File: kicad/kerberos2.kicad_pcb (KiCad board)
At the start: 2 copper layers, 62.5 x 83.8 mm, 15 parts, among them J1 USB4125-GF-A_REVA2, J2 MIDI-in, J3 MIDI-thru, J4 MIDI-out, SW1 TL1105JAF160Q, U1 RP2040, U2 W9812G6KH-6, U3 T8Q144, U4 MX25L25645G

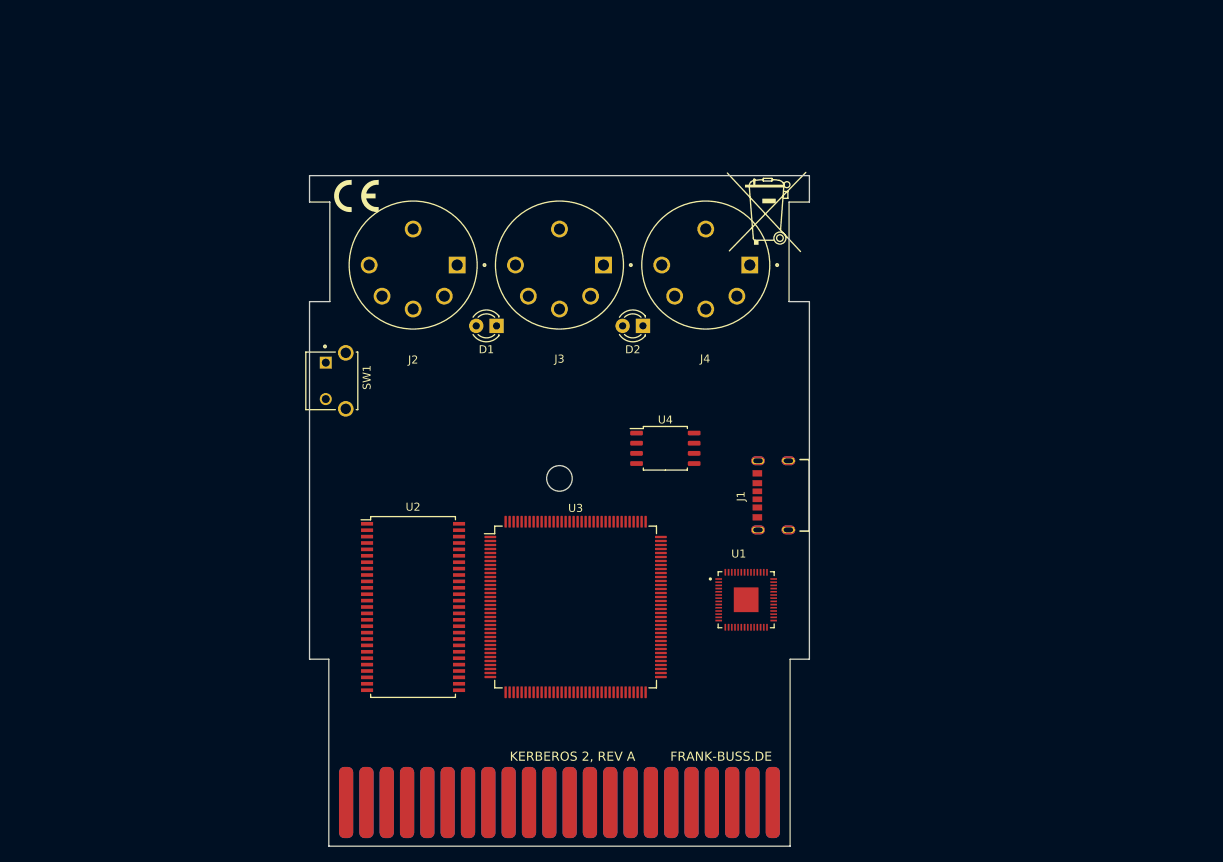
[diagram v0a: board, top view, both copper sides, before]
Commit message: first complete test version for Kerberos 2
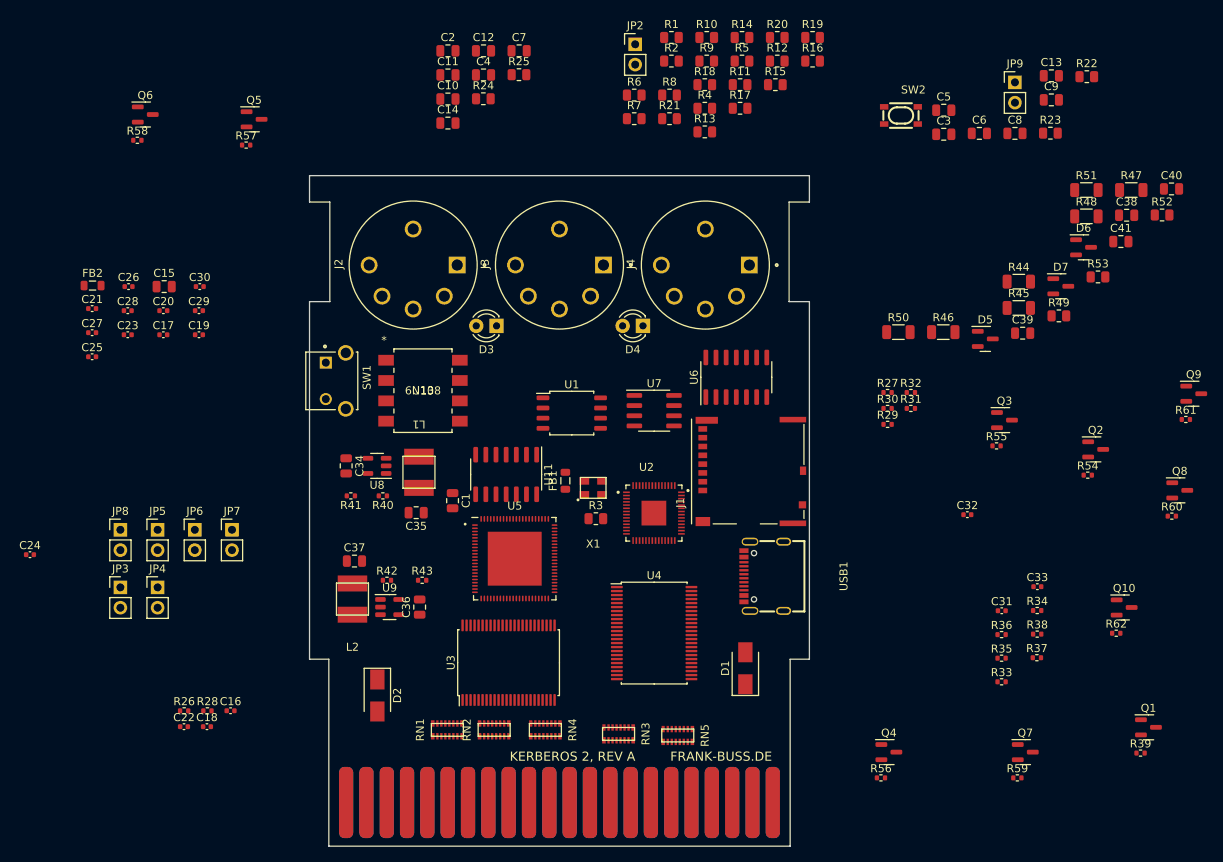
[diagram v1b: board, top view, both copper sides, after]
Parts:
- removed @HOLE0: , 
- removed U$1: , midi:CE-4MM
- removed U$2: , midi:MUELLTONNE_10.00
- removed the U1 at (100.4, 92.0)
- added C1: 100n, Capacitor_SMD:C_0805_2012Metric, F.Cu at (63.7, 79.7)
- added C10: 100n, Capacitor_SMD:C_0805_2012Metric, F.Cu at (63.1, 29.4)
- added C11: 100n, Capacitor_SMD:C_0805_2012Metric, F.Cu at (63.1, 26.4)
- added C12: 100n, Capacitor_SMD:C_0805_2012Metric, F.Cu at (67.6, 23.4)
- added C13: 100n, Capacitor_SMD:C_0805_2012Metric, F.Cu at (138.6, 26.5)
- added C14: 1u, Capacitor_SMD:C_0805_2012Metric, F.Cu at (63.1, 32.5)
- added C15: 4.7u, Capacitor_SMD:C_0805_2012Metric, F.Cu at (27.6, 52.9)
- added C16: 100n, Capacitor_SMD:C_0402_1005Metric, F.Cu at (36.0, 105.9)
- added C17: 100n, Capacitor_SMD:C_0402_1005Metric, F.Cu at (27.6, 58.9)
- added C18: 100n, Capacitor_SMD:C_0402_1005Metric, F.Cu at (33.0, 107.9)
- added C19: 100n, Capacitor_SMD:C_0402_1005Metric, F.Cu at (32.0, 58.9)
- added C2: 10u, Capacitor_SMD:C_0805_2012Metric, F.Cu at (63.1, 23.4)
- added C20: 100n, Capacitor_SMD:C_0402_1005Metric, F.Cu at (27.6, 55.9)
- added C21: 100n, Capacitor_SMD:C_0402_1005Metric, F.Cu at (18.6, 55.6)
- added C22: 100n, Capacitor_SMD:C_0402_1005Metric, F.Cu at (30.1, 107.9)
- added C23: 100n, Capacitor_SMD:C_0402_1005Metric, F.Cu at (23.1, 58.9)
- added C24: 100n, Capacitor_SMD:C_0402_1005Metric, F.Cu at (10.9, 86.4)
- added C25: 100n, Capacitor_SMD:C_0402_1005Metric, F.Cu at (18.6, 61.7)
- added C26: 100n, Capacitor_SMD:C_0402_1005Metric, F.Cu at (23.2, 52.9)
- added C27: 100n, Capacitor_SMD:C_0402_1005Metric, F.Cu at (18.6, 58.6)
- added C28: 100n, Capacitor_SMD:C_0402_1005Metric, F.Cu at (23.1, 55.9)
- added C29: 100n, Capacitor_SMD:C_0402_1005Metric, F.Cu at (32.0, 55.9)
- added C3: 100n, Capacitor_SMD:C_0805_2012Metric, F.Cu at (125.1, 33.9)
- added C30: 100n, Capacitor_SMD:C_0402_1005Metric, F.Cu at (32.1, 52.9)
- added C31: 100n, Capacitor_SMD:C_0402_1005Metric, F.Cu at (132.3, 93.4)
- added C32: 100n, Capacitor_SMD:C_0402_1005Metric, F.Cu at (128.1, 81.4)
- added C33: 100n, Capacitor_SMD:C_0402_1005Metric, F.Cu at (136.8, 90.4)
- added C34: 4.7u, Capacitor_SMD:C_0805_2012Metric, F.Cu at (50.4, 75.3)
- added C35: 10u, Capacitor_SMD:C_0805_2012Metric, F.Cu at (59.1, 81.2)
- added C36: 4.7u, Capacitor_SMD:C_0805_2012Metric, F.Cu at (59.6, 93.0)
- added C37: 10u, Capacitor_SMD:C_0805_2012Metric, F.Cu at (51.4, 87.2)
- added C38: 1n, Capacitor_SMD:C_0805_2012Metric, F.Cu at (148.0, 44.0)
- added C39: 1n, Capacitor_SMD:C_0805_2012Metric, F.Cu at (135.0, 58.7)
- added C4: 100n, Capacitor_SMD:C_0805_2012Metric, F.Cu at (67.6, 26.4)
- added C40: 100n, Capacitor_SMD:C_0805_2012Metric, F.Cu at (153.6, 40.7)
- added C41: 100n, Capacitor_SMD:C_0805_2012Metric, F.Cu at (147.2, 47.3)
- added C5: 100n, Capacitor_SMD:C_0805_2012Metric, F.Cu at (125.1, 30.8)
- added C6: 100n, Capacitor_SMD:C_0805_2012Metric, F.Cu at (129.6, 33.7)
- added C7: 100n, Capacitor_SMD:C_0805_2012Metric, F.Cu at (72.0, 23.4)
- added C8: 100n, Capacitor_SMD:C_0805_2012Metric, F.Cu at (134.0, 33.7)
- added C9: 1u, Capacitor_SMD:C_0805_2012Metric, F.Cu at (138.6, 29.6)
- added D3: ~, LED_THT:LED_D3.0mm, F.Cu at (69.2, 57.8)
- added D4: ~, LED_THT:LED_D3.0mm, F.Cu at (87.5, 57.8)
- added D5: BAV99, Package_TO_SOT_SMD:SOT-23, F.Cu at (130.3, 59.4)
- added D6: BAV99, Package_TO_SOT_SMD:SOT-23, F.Cu at (142.6, 48.0)
- added D7: BAV99, Package_TO_SOT_SMD:SOT-23, F.Cu at (139.7, 52.9)
- added FB1: FerriteBead, Inductor_SMD:L_0805_2012Metric, F.Cu at (77.8, 77.2)
- added FB2: FerriteBead, Inductor_SMD:L_0805_2012Metric, F.Cu at (18.7, 52.8)
- added JP2: host-mode-supply, Connector_PinHeader_2.54mm:PinHeader_1x02_P2.54mm_Vertical, F.Cu at (86.5, 22.6)
- added JP3: 3.3V+, Connector_PinHeader_2.54mm:PinHeader_1x02_P2.54mm_Vertical, F.Cu at (22.2, 90.5)
- added JP4: 3.3V, Connector_PinHeader_2.54mm:PinHeader_1x02_P2.54mm_Vertical, F.Cu at (26.8, 90.5)
- added JP5: 3.3V-, Connector_PinHeader_2.54mm:PinHeader_1x02_P2.54mm_Vertical, F.Cu at (26.8, 83.3)
- added JP6: 1.2V+, Connector_PinHeader_2.54mm:PinHeader_1x02_P2.54mm_Vertical, F.Cu at (31.5, 83.3)
- added JP7: 1.2V, Connector_PinHeader_2.54mm:PinHeader_1x02_P2.54mm_Vertical, F.Cu at (36.1, 83.3)
- added JP8: 1.2V-, Connector_PinHeader_2.54mm:PinHeader_1x02_P2.54mm_Vertical, F.Cu at (22.2, 83.3)
- added JP9: ~{USB_BOOT}, Connector_PinHeader_2.54mm:PinHeader_1x02_P2.54mm_Vertical, F.Cu at (134.0, 27.4)
- added L1: 4.7u, coil:coil, F.Cu at (59.5, 76.1)
- added L2: 4.7u, coil:coil, F.Cu at (51.2, 92.0)
- added Q1: Q_NMOS_GSD, Package_TO_SOT_SMD:SOT-23, F.Cu at (150.7, 108.0)
- added Q10: Q_NMOS_GSD, Package_TO_SOT_SMD:SOT-23, F.Cu at (147.7, 93.0)
- added Q2: Q_NMOS_GSD, Package_TO_SOT_SMD:SOT-23, F.Cu at (144.1, 73.2)
- added Q3: Q_NMOS_GSD, Package_TO_SOT_SMD:SOT-23, F.Cu at (132.7, 69.6)
- added Q4: Q_NMOS_GSD, Package_TO_SOT_SMD:SOT-23, F.Cu at (118.2, 111.1)
- added Q5: Q_NMOS_GSD, Package_TO_SOT_SMD:SOT-23, F.Cu at (38.9, 32.0)
- added Q6: Q_NMOS_GSD, Package_TO_SOT_SMD:SOT-23, F.Cu at (25.3, 31.4)
- added Q7: Q_NMOS_GSD, Package_TO_SOT_SMD:SOT-23, F.Cu at (135.3, 111.1)
- added Q8: Q_NMOS_GSD, Package_TO_SOT_SMD:SOT-23, F.Cu at (154.6, 78.4)
- added Q9: Q_NMOS_GSD, Package_TO_SOT_SMD:SOT-23, F.Cu at (156.3, 66.3)
- added R1: 5.1, Resistor_SMD:R_0805_2012Metric, F.Cu at (91.1, 21.8)
- added R10: 22, Resistor_SMD:R_0805_2012Metric, F.Cu at (95.5, 21.8)
- added R11: 22, Resistor_SMD:R_0805_2012Metric, F.Cu at (99.6, 27.6)
- added R12: 22, Resistor_SMD:R_0805_2012Metric, F.Cu at (104.3, 24.7)
- added R13: 22, Resistor_SMD:R_0805_2012Metric, F.Cu at (95.2, 33.5)
- added R14: 22, Resistor_SMD:R_0805_2012Metric, F.Cu at (99.9, 21.8)
- added R15: 22, Resistor_SMD:R_0805_2012Metric, F.Cu at (104.0, 27.6)
- added R16: 22, Resistor_SMD:R_0805_2012Metric, F.Cu at (108.7, 24.7)
- added R17: 22, Resistor_SMD:R_0805_2012Metric, F.Cu at (99.6, 30.6)
- added R18: 22, Resistor_SMD:R_0805_2012Metric, F.Cu at (95.2, 27.6)
- added R19: 22, Resistor_SMD:R_0805_2012Metric, F.Cu at (108.7, 21.8)
- added R2: 5.1, Resistor_SMD:R_0805_2012Metric, F.Cu at (91.1, 24.7)
- added R20: 1k, Resistor_SMD:R_0805_2012Metric, F.Cu at (104.3, 21.8)
- added R21: 1k, Resistor_SMD:R_0805_2012Metric, F.Cu at (90.8, 31.9)
- added R22: 10k, Resistor_SMD:R_0805_2012Metric, F.Cu at (143.0, 26.6)
- added R23: 10k, Resistor_SMD:R_0805_2012Metric, F.Cu at (138.4, 33.7)
- added R24: 1k, Resistor_SMD:R_0805_2012Metric, F.Cu at (67.5, 29.4)
- added R25: 10k, Resistor_SMD:R_0805_2012Metric, F.Cu at (72.0, 26.4)
- added R26: 10k, Resistor_SMD:R_0402_1005Metric, F.Cu at (30.1, 105.9)
- added R27: 10k, Resistor_SMD:R_0402_1005Metric, F.Cu at (118.1, 66.1)
- added R28: 10k, Resistor_SMD:R_0402_1005Metric, F.Cu at (33.1, 105.9)
- added R29: 10k, Resistor_SMD:R_0402_1005Metric, F.Cu at (118.1, 70.1)
- added R3: 27, Resistor_SMD:R_0805_2012Metric, F.Cu at (81.6, 81.9)
- added R30: 10k, Resistor_SMD:R_0402_1005Metric, F.Cu at (118.1, 68.1)
- added R31: 10k, Resistor_SMD:R_0402_1005Metric, F.Cu at (121.0, 68.1)
- added R32: 10k, Resistor_SMD:R_0402_1005Metric, F.Cu at (121.0, 66.1)
- added R33: 10k, Resistor_SMD:R_0402_1005Metric, F.Cu at (132.3, 102.3)
- added R34: 10k, Resistor_SMD:R_0402_1005Metric, F.Cu at (136.8, 93.4)
- added R35: 1k, Resistor_SMD:R_0402_1005Metric, F.Cu at (132.3, 99.3)
- added R36: 1k, Resistor_SMD:R_0402_1005Metric, F.Cu at (132.3, 96.4)
- added R37: 10k, Resistor_SMD:R_0402_1005Metric, F.Cu at (136.7, 99.3)
- added R38: 10k, Resistor_SMD:R_0402_1005Metric, F.Cu at (136.8, 96.3)
- added R39: 10k, Resistor_SMD:R_0402_1005Metric, F.Cu at (149.7, 111.2)
- added R4: 27, Resistor_SMD:R_0805_2012Metric, F.Cu at (95.2, 30.6)
- added R40: R, Resistor_SMD:R_0402_1005Metric, F.Cu at (55.0, 79.0)
- added R41: R, Resistor_SMD:R_0402_1005Metric, F.Cu at (51.0, 79.0)
- added R42: R, Resistor_SMD:R_0402_1005Metric, F.Cu at (55.5, 89.6)
- added R43: R, Resistor_SMD:R_0402_1005Metric, F.Cu at (59.9, 89.6)
- added R44: 220, Resistor_SMD:R_1206_3216Metric, F.Cu at (134.5, 52.3)
- added R45: 220, Resistor_SMD:R_1206_3216Metric, F.Cu at (134.5, 55.6)
- added R46: 220, Resistor_SMD:R_1206_3216Metric, F.Cu at (125.0, 58.6)
- added R47: 220, Resistor_SMD:R_1206_3216Metric, F.Cu at (148.5, 40.8)
- added R48: 220, Resistor_SMD:R_1206_3216Metric, F.Cu at (142.9, 44.1)
- added R49: 10k, Resistor_SMD:R_0805_2012Metric, F.Cu at (139.5, 56.5)
- added R5: 27, Resistor_SMD:R_0805_2012Metric, F.Cu at (99.9, 24.7)
- added R50: 220, Resistor_SMD:R_1206_3216Metric, F.Cu at (119.4, 58.6)
- added R51: 220, Resistor_SMD:R_1206_3216Metric, F.Cu at (142.9, 40.8)
- added R52: 1k8, Resistor_SMD:R_0805_2012Metric, F.Cu at (152.4, 43.9)
- added R53: 3k3, Resistor_SMD:R_0805_2012Metric, F.Cu at (144.4, 51.7)
- added R54: 10k, Resistor_SMD:R_0402_1005Metric, F.Cu at (143.1, 76.5)
- added R55: 10k, Resistor_SMD:R_0402_1005Metric, F.Cu at (131.7, 72.8)
- added R56: 10k, Resistor_SMD:R_0402_1005Metric, F.Cu at (117.2, 114.3)
- added R57: 10k, Resistor_SMD:R_0402_1005Metric, F.Cu at (37.9, 35.2)
- added R58: 10k, Resistor_SMD:R_0402_1005Metric, F.Cu at (24.3, 34.6)
- added R59: 10k, Resistor_SMD:R_0402_1005Metric, F.Cu at (134.3, 114.3)
- added R6: 27, Resistor_SMD:R_0805_2012Metric, F.Cu at (86.4, 28.9)
- added R60: 10k, Resistor_SMD:R_0402_1005Metric, F.Cu at (153.6, 81.6)
- added R61: 10k, Resistor_SMD:R_0402_1005Metric, F.Cu at (155.4, 69.5)
- added R62: 10k, Resistor_SMD:R_0402_1005Metric, F.Cu at (146.7, 96.2)
- added R7: 22, Resistor_SMD:R_0805_2012Metric, F.Cu at (86.4, 31.9)
- added R8: 22, Resistor_SMD:R_0805_2012Metric, F.Cu at (90.8, 28.9)
- added R9: 22, Resistor_SMD:R_0805_2012Metric, F.Cu at (95.5, 24.7)
- added RN1: 33, resistor-network:16P8, F.Cu at (63.0, 108.3)
- added RN2: 33, resistor-network:16P8, F.Cu at (68.9, 108.3)
- added RN3: 33, resistor-network:16P8, F.Cu at (84.5, 108.8)
- added RN4: 33, resistor-network:16P8, F.Cu at (75.3, 108.3)
- added RN5: 33, resistor-network:16P8, F.Cu at (91.8, 109.0)
- added SW2: SKRPADE010, button:KEY-SMD_4P-L4.2-W3.2-P2.20-LS4.6, F.Cu at (119.8, 31.5)
- added U10: 6N138, 6N138S:6N138S, F.Cu at (60.0, 65.9)
- added U11: 74LS14, Package_SO:SOIC-14_3.9x8.7mm_P1.27mm, F.Cu at (70.4, 76.4)
- added U4: 74ALVC164245DGG,51, Package_SO:TSSOP-48_8x12.5mm_P0.5mm, F.Cu at (88.9, 96.2)
- added U5: GW1NR-4&4B_QN881, qn88:QFN-88_EP_10x10_Pitch0.4mm, F.Cu at (71.5, 86.9)
- added U6: AD8694ARZ, Package_SO:SOIC-14_3.9x8.7mm_P1.27mm, F.Cu at (99.2, 64.2)
- added U7: TMCS1108A3UQDR, Package_SO:SOIC-8_3.9x4.9mm_P1.27mm, F.Cu at (88.9, 68.4)
- added U8: M3406, Package_TO_SOT_SMD:TSOT-23-5, F.Cu at (54.3, 75.3)
- added U9: M3406, Package_TO_SOT_SMD:TSOT-23-5, F.Cu at (55.8, 93.0)
- added USB1: TYPEC-304J-BCP16, usb-c:USB-C-SMD_TYPEC-304J-BCP16, F.Cu at (102.6, 89.1)
- added X1: SX3M12.000M20F30TNN, oscillator:SX3M12.000M20F30TNN, F.Cu at (81.3, 78.0)
- D1, D2: value LED -> D_Schottky; footprint LED_THT:LED_D3.0mm -> Diode_SMD:D_SMA
- J1: value USB4125-GF-A_REVA2 -> 503398-1892; footprint usb-c:GCT_USB4125-GF-A_REVA2 -> sd-card:MOLEX_503398-1892
- SW1: value TL1105JAF160Q -> side-button
- U2: value W9812G6KH-6 -> RP2040; footprint Package_SO:TSOP-II-54_22.2x10.16mm_P0.8mm -> rp2040:QFN40P700X700X90-57N
- U3: value T8Q144 -> 74ALVC164245DGG,51; footprint Package_QFP:LQFP-144_20x20mm_P0.5mm -> Package_SO:TSSOP-48_8x12.5mm_P0.5mm
- moved D2 56.9 mm to (54.3, 104.0), turned to -90 degrees
- moved D1 52.9 mm to (100.3, 100.6), turned to 90 degrees
- moved U2 32.3 mm to (88.9, 81.2)
- moved U1 12.5 mm to (78.6, 68.7)
- moved U3 10.9 mm to (70.7, 99.9), turned to 90 degrees
- moved J1 5.22 mm to (100.6, 76.0)
- moved J4 0.05 mm to (95.3, 50.2)
- renumbered U4 to U1
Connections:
- D1 pad 1: unconnected-(D1-Pad1) -> +5V
- D1 pad 2: unconnected-(D1-Pad2) -> Net-(D1-Pad2)
- D2 pad 1: unconnected-(D2-Pad1) -> +5V
- D2 pad 2: unconnected-(D2-Pad2) -> Net-(D2-Pad2)
- J2 pad 4: unconnected-(J2-Pad4) -> Net-(J2-Pad4)
- J2 pad 5: unconnected-(J2-Pad5) -> Net-(D5-Pad1)
- J3 pad 2: unconnected-(J3-Pad2) -> GND
- J3 pad 4: unconnected-(J3-Pad4) -> Net-(J3-Pad4)
- J3 pad 5: unconnected-(J3-Pad5) -> Net-(C38-Pad1)
- J3 pad S: unconnected-(J3-PadS) -> GND
- J4 pad 2: unconnected-(J4-Pad2) -> GND
- J4 pad 4: unconnected-(J4-Pad4) -> Net-(J4-Pad4)
- J4 pad 5: unconnected-(J4-Pad5) -> Net-(C39-Pad1)
- J4 pad S: unconnected-(J4-PadS) -> GND
- JP1 pad 1: unconnected-(JP1-Pad1) -> GND
- JP1 pad 10: unconnected-(JP1-Pad10) -> Net-(JP1-Pad10)
- JP1 pad 11: unconnected-(JP1-Pad11) -> Net-(JP1-Pad11)
- JP1 pad 12: unconnected-(JP1-Pad12) -> Net-(JP1-Pad12)
- JP1 pad 13: unconnected-(JP1-Pad13) -> Net-(JP1-Pad13)
- JP1 pad 14: unconnected-(JP1-Pad14) -> Net-(JP1-Pad14)
- JP1 pad 15: unconnected-(JP1-Pad15) -> Net-(JP1-Pad15)
- JP1 pad 16: unconnected-(JP1-Pad16) -> Net-(JP1-Pad16)
- JP1 pad 17: unconnected-(JP1-Pad17) -> Net-(JP1-Pad17)
- JP1 pad 18: unconnected-(JP1-Pad18) -> Net-(JP1-Pad18)
- JP1 pad 19: unconnected-(JP1-Pad19) -> Net-(JP1-Pad19)
- JP1 pad 2: unconnected-(JP1-Pad2) -> Net-(D2-Pad2)
- JP1 pad 20: unconnected-(JP1-Pad20) -> Net-(JP1-Pad20)
- JP1 pad 21: unconnected-(JP1-Pad21) -> Net-(JP1-Pad21)
- JP1 pad 22: unconnected-(JP1-Pad22) -> GND
- JP1 pad 3: unconnected-(JP1-Pad3) -> Net-(D2-Pad2)
- JP1 pad 4: unconnected-(JP1-Pad4) -> Net-(JP1-Pad4)
- JP1 pad 5: unconnected-(JP1-Pad5) -> Net-(JP1-Pad5)
- JP1 pad 6: unconnected-(JP1-Pad6) -> Net-(JP1-Pad6)
- JP1 pad 7: unconnected-(JP1-Pad7) -> Net-(JP1-Pad7)
- JP1 pad 8: unconnected-(JP1-Pad8) -> Net-(JP1-Pad8)
- JP1 pad 9: unconnected-(JP1-Pad9) -> Net-(JP1-Pad9)
- JP1 pad A: unconnected-(JP1-PadA) -> GND
- JP1 pad B: unconnected-(JP1-PadB) -> Net-(JP1-PadB)
- JP1 pad C: unconnected-(JP1-PadC) -> Net-(JP1-PadC)
- JP1 pad D: unconnected-(JP1-PadD) -> Net-(JP1-PadD)
- JP1 pad E: unconnected-(JP1-PadE) -> Net-(JP1-PadE)
- JP1 pad F: unconnected-(JP1-PadF) -> Net-(JP1-PadF)
- JP1 pad H: unconnected-(JP1-PadH) -> Net-(JP1-PadH)
- JP1 pad J: unconnected-(JP1-PadJ) -> Net-(JP1-PadJ)
- JP1 pad K: unconnected-(JP1-PadK) -> Net-(JP1-PadK)
- JP1 pad L: unconnected-(JP1-PadL) -> Net-(JP1-PadL)
- JP1 pad M: unconnected-(JP1-PadM) -> Net-(JP1-PadM)
- JP1 pad N: unconnected-(JP1-PadN) -> Net-(JP1-PadN)
- JP1 pad P: unconnected-(JP1-PadP) -> Net-(JP1-PadP)
- JP1 pad R: unconnected-(JP1-PadR) -> Net-(JP1-PadR)
- JP1 pad S: unconnected-(JP1-PadS) -> Net-(JP1-PadS)
- JP1 pad T: unconnected-(JP1-PadT) -> Net-(JP1-PadT)
- JP1 pad U: unconnected-(JP1-PadU) -> Net-(JP1-PadU)
- JP1 pad V: unconnected-(JP1-PadV) -> Net-(JP1-PadV)
- JP1 pad W: unconnected-(JP1-PadW) -> Net-(JP1-PadW)
- JP1 pad X: unconnected-(JP1-PadX) -> Net-(JP1-PadX)
- JP1 pad Y: unconnected-(JP1-PadY) -> Net-(JP1-PadY)
- JP1 pad Z: unconnected-(JP1-PadZ) -> GND
- SW1 pad 1: unconnected-(SW1-Pad1) -> GND
- SW1 pad 2: unconnected-(SW1-Pad2) -> Net-(R22-Pad2)
- U1 pad 1: unconnected-(U4-Pad1) -> /GW1NR FPGA/FLASH_CS
- U1 pad 2: unconnected-(U4-Pad2) -> /GW1NR FPGA/FLASH-SIO1
- U1 pad 3: unconnected-(U4-Pad3) -> /GW1NR FPGA/FLASH-SIO2
- U1 pad 4: unconnected-(U4-Pad4) -> GND
- U1 pad 5: unconnected-(U4-Pad5) -> /GW1NR FPGA/FLASH-SIO0
- U1 pad 6: unconnected-(U4-Pad6) -> /GW1NR FPGA/FLASH-SCLK
- U1 pad 7: unconnected-(U4-Pad7) -> /GW1NR FPGA/FLASH-SIO3
- U1 pad 8: unconnected-(U4-Pad8) -> +3.3V
- U2 pad 1: Net-(U2-Pad1) -> +3.3V
- U2 pad 10: unconnected-(U2-Pad10) -> +3.3V
- U2 pad 11: unconnected-(U2-Pad11) -> /RP2040 microcontroller/spare2
- U2 pad 12: Net-(U2-Pad12) -> /RP2040 microcontroller/spare3
- U2 pad 13: unconnected-(U2-Pad13) -> /RP2040 microcontroller/spare4
- U2 pad 14: Net-(U2-Pad1) -> /RP2040 microcontroller/spare5
- U2 pad 15: unconnected-(U2-Pad15) -> /RP2040 microcontroller/spare6
- U2 pad 16: unconnected-(U2-Pad16) -> Net-(R22-Pad2)
- U2 pad 19: unconnected-(U2-Pad19) -> GND
- U2 pad 2: unconnected-(U2-Pad2) -> /RP2040 microcontroller/JTAGSEL_N
- U2 pad 20: unconnected-(U2-Pad20) -> /RP2040 microcontroller/XIN
- U2 pad 22: unconnected-(U2-Pad22) -> +3.3V
- U2 pad 23: unconnected-(U2-Pad23) -> /RP2040 microcontroller/1.1V
- U2 pad 26: unconnected-(U2-Pad26) -> Net-(R23-Pad1)
- U2 pad 27: Net-(U2-Pad1) -> unconnected-(U2-Pad27)
- U2 pad 28: Net-(U2-Pad28) -> unconnected-(U2-Pad28)
- U2 pad 3: Net-(U2-Pad3) -> /RP2040 microcontroller/TCK
- U2 pad 30: unconnected-(U2-Pad30) -> Net-(J1-Pad3)
- U2 pad 31: unconnected-(U2-Pad31) -> Net-(J1-Pad5)
- U2 pad 32: unconnected-(U2-Pad32) -> Net-(J1-Pad7)
- U2 pad 33: unconnected-(U2-Pad33) -> +3.3V
- U2 pad 34: unconnected-(U2-Pad34) -> Net-(J1-Pad8)
- U2 pad 35: unconnected-(U2-Pad35) -> Net-(J1-Pad1)
- U2 pad 36: unconnected-(U2-Pad36) -> Net-(J1-Pad2)
- U2 pad 37: unconnected-(U2-Pad37) -> Net-(J1-Pad10)
- U2 pad 4: unconnected-(U2-Pad4) -> /RP2040 microcontroller/TMS
- U2 pad 41: Net-(U2-Pad28) -> unconnected-(U2-Pad41)
- U2 pad 42: unconnected-(U2-Pad42) -> +3.3V
- U2 pad 43: Net-(U2-Pad3) -> +3.3V
- U2 pad 44: unconnected-(U2-Pad44) -> +3.3V
- U2 pad 45: unconnected-(U2-Pad45) -> /RP2040 microcontroller/1.1V
- U2 pad 46: Net-(U2-Pad12) -> /RP2040 microcontroller/USB_D-
- U2 pad 47: unconnected-(U2-Pad47) -> /RP2040 microcontroller/USB_D+
- U2 pad 48: unconnected-(U2-Pad48) -> +3.3V
- U2 pad 49: Net-(U2-Pad3) -> +3.3V
- U2 pad 5: unconnected-(U2-Pad5) -> /RP2040 microcontroller/TDO
- U2 pad 50: unconnected-(U2-Pad50) -> /RP2040 microcontroller/1.1V
- U2 pad 51: unconnected-(U2-Pad51) -> /GW1NR FPGA/FLASH-SIO3
- U2 pad 52: Net-(U2-Pad12) -> /GW1NR FPGA/FLASH-SCLK
- U2 pad 53: unconnected-(U2-Pad53) -> /GW1NR FPGA/FLASH-SIO0
- U2 pad 54: Net-(U2-Pad28) -> /GW1NR FPGA/FLASH-SIO2
- U2 pad 6: Net-(U2-Pad12) -> /RP2040 microcontroller/TDI
- U2 pad 7: unconnected-(U2-Pad7) -> /RP2040 microcontroller/DONE
- U2 pad 8: unconnected-(U2-Pad8) -> /RP2040 microcontroller/RECONFIG_N
- U2 pad 9: Net-(U2-Pad3) -> /RP2040 microcontroller/spare1
- U3 pad 1: unconnected-(U3-Pad1) -> /GW1NR FPGA/DIR_A
- U3 pad 10: unconnected-(U3-Pad10) -> GND
- U3 pad 11: unconnected-(U3-Pad11) -> /GW1NR FPGA/A6
- U3 pad 12: unconnected-(U3-Pad12) -> /GW1NR FPGA/A7
- U3 pad 13: unconnected-(U3-Pad13) -> /GW1NR FPGA/A8
- U3 pad 14: unconnected-(U3-Pad14) -> /GW1NR FPGA/A9
- U3 pad 15: unconnected-(U3-Pad15) -> GND
- U3 pad 16: unconnected-(U3-Pad16) -> /GW1NR FPGA/A10
- U3 pad 17: unconnected-(U3-Pad17) -> /GW1NR FPGA/A11
- U3 pad 18: unconnected-(U3-Pad18) -> +5V
- U3 pad 19: unconnected-(U3-Pad19) -> /GW1NR FPGA/A12
- U3 pad 2: unconnected-(U3-Pad2) -> /GW1NR FPGA/A0
- U3 pad 20: unconnected-(U3-Pad20) -> /GW1NR FPGA/A13
- U3 pad 21: unconnected-(U3-Pad21) -> GND
- U3 pad 22: unconnected-(U3-Pad22) -> /GW1NR FPGA/A14
- U3 pad 23: unconnected-(U3-Pad23) -> /GW1NR FPGA/A15
- U3 pad 24: unconnected-(U3-Pad24) -> /GW1NR FPGA/DIR_A
- U3 pad 25: unconnected-(U3-Pad25) -> GND
- U3 pad 26: unconnected-(U3-Pad26) -> /GW1NR FPGA/A15_t
- U3 pad 27: unconnected-(U3-Pad27) -> /GW1NR FPGA/A14_t
- U3 pad 28: unconnected-(U3-Pad28) -> GND
- U3 pad 29: unconnected-(U3-Pad29) -> /GW1NR FPGA/A13_t
- U3 pad 3: unconnected-(U3-Pad3) -> /GW1NR FPGA/A1
- U3 pad 30: unconnected-(U3-Pad30) -> /GW1NR FPGA/A12_t
- U3 pad 31: unconnected-(U3-Pad31) -> +3.3V
- U3 pad 32: unconnected-(U3-Pad32) -> /GW1NR FPGA/A11_t
- U3 pad 33: unconnected-(U3-Pad33) -> /GW1NR FPGA/A10_t
- U3 pad 34: unconnected-(U3-Pad34) -> GND
- U3 pad 35: unconnected-(U3-Pad35) -> /GW1NR FPGA/A9_t
- U3 pad 36: unconnected-(U3-Pad36) -> /GW1NR FPGA/A8_t
- U3 pad 37: unconnected-(U3-Pad37) -> /GW1NR FPGA/A7_t
- U3 pad 38: unconnected-(U3-Pad38) -> /GW1NR FPGA/A6_t
- U3 pad 39: unconnected-(U3-Pad39) -> GND
- U3 pad 4: unconnected-(U3-Pad4) -> GND
- U3 pad 40: unconnected-(U3-Pad40) -> /GW1NR FPGA/A5_t
- U3 pad 41: unconnected-(U3-Pad41) -> /GW1NR FPGA/A4_t
- U3 pad 42: unconnected-(U3-Pad42) -> +3.3V
- U3 pad 43: unconnected-(U3-Pad43) -> /GW1NR FPGA/A3_t
- U3 pad 44: unconnected-(U3-Pad44) -> /GW1NR FPGA/A2_t
- U3 pad 45: unconnected-(U3-Pad45) -> GND
- U3 pad 46: unconnected-(U3-Pad46) -> /GW1NR FPGA/A1_t
- U3 pad 47: unconnected-(U3-Pad47) -> /GW1NR FPGA/A0_t
- U3 pad 48: unconnected-(U3-Pad48) -> GND
- U3 pad 5: unconnected-(U3-Pad5) -> /GW1NR FPGA/A2
- U3 pad 6: unconnected-(U3-Pad6) -> /GW1NR FPGA/A3
- U3 pad 7: unconnected-(U3-Pad7) -> +5V
- U3 pad 8: unconnected-(U3-Pad8) -> /GW1NR FPGA/A4
- U3 pad 9: unconnected-(U3-Pad9) -> /GW1NR FPGA/A5
